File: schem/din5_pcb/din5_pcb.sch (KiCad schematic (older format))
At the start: 74 parts, among them J1 Conn_01x03_Male, J101 DIN-5_180degree, J102 DIN-5_180degree, J103 DIN-5_180degree, J104 DIN-5_180degree, J111 do not equip, J112 do not equip, J113 do not equip, J114 do not equip, J2 Conn_02x03_Odd_Even, J201 DIN-5_180degree, J202 DIN-5_180degree, J203 DIN-5_180degree, J204 DIN-5_180degree, J211 do not equip, J212 do not equip, J213 do not equip, J214 do not equip, J3 Conn_02x03_Odd_Even, J4 USB_B_Micro, J5 USB_B_Micro, J6 Conn_02x02_Odd_Even, J7 Conn_02x02_Odd_Even, U1 74HCT245, U101 HCPL-2630, U102 HCPL-2630, U2 74HC595, U3 74HC165

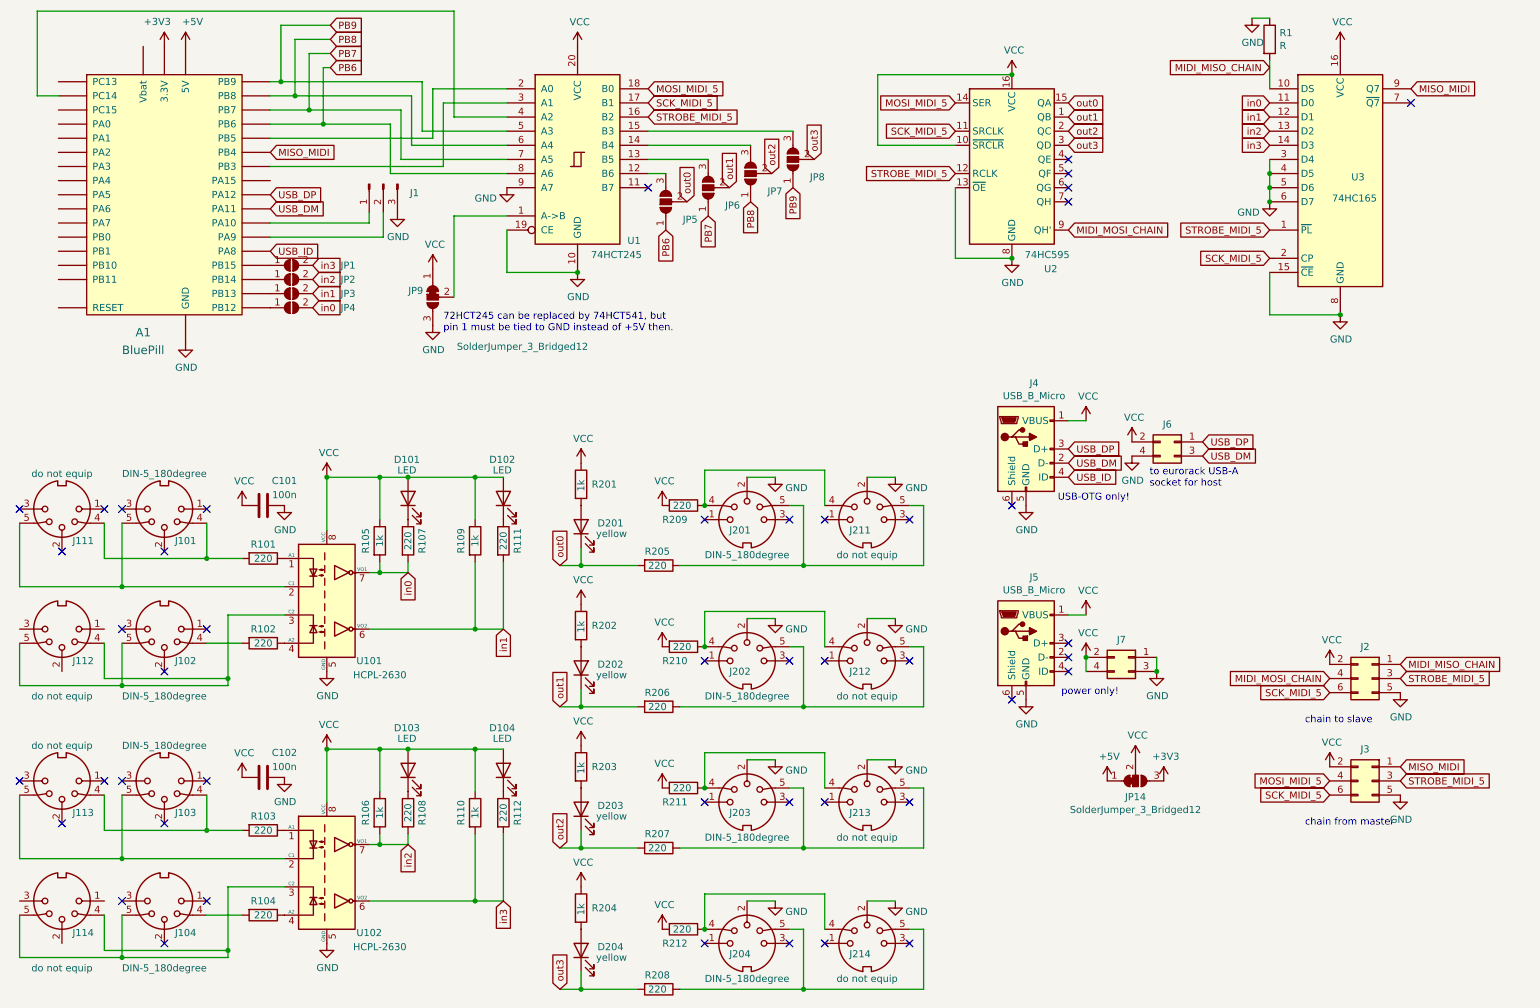
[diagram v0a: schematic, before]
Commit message: din 5 pin pcb finished. todo: autoroute
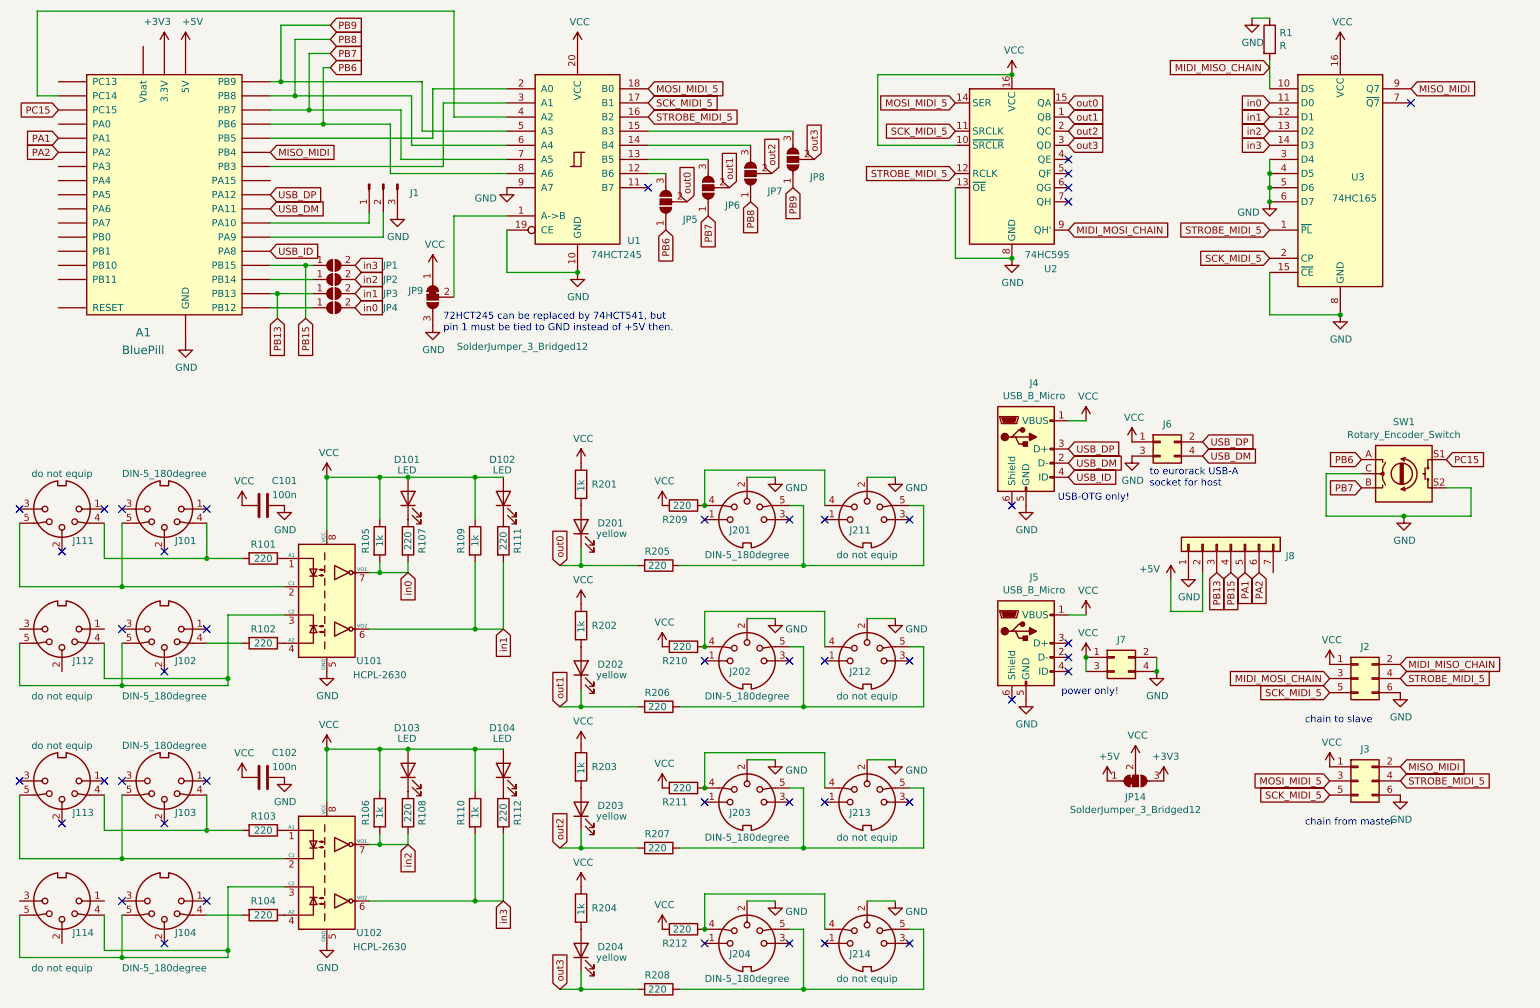
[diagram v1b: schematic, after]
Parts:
- added J8: Conn_01x07, Connector_PinHeader_2.54mm:PinHeader_1x07_P2.54mm_Vertical, symbol Connector_Generic:Conn_01x07
- added SW1: Rotary_Encoder_Switch, Rotary_Encoder:RotaryEncoder_Alps_EC11E-Switch_Vertical_H20mm, symbol Device:Rotary_Encoder_Switch
- J2, J3: footprint Connector_PinSocket_2.54mm:PinSocket_2x03_P2.54mm_Vertical -> Connector_PinHeader_2.54mm:PinHeader_2x03_P2.54mm_Vertical
- J6, J7: footprint Connector_PinSocket_2.54mm:PinSocket_2x02_P2.54mm_Vertical -> Connector_PinHeader_2.54mm:PinHeader_2x02_P2.54mm_Vertical
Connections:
- net +5V: now also J8.2 (Pin_2)
- net GND: now also J2.6 (Pin_6), J3.6 (Pin_6), J6.3 (Pin_3), J7.2 (Pin_2), J7.4 (Pin_4), J8.1 (Pin_1), SW1.C, SW1.S2; no longer J2.5 (Pin_5), J3.5 (Pin_5), J6.4 (Pin_4), J7.1 (Pin_1), J7.3 (Pin_3)
- net MIDI_MISO_CHAIN: now also J2.2 (Pin_2); no longer J2.1 (Pin_1)
- net MIDI_MOSI_CHAIN: now also J2.3 (Pin_3); no longer J2.4 (Pin_4)
- net MISO_MIDI: now also J3.2 (Pin_2); no longer J3.1 (Pin_1)
- net MOSI_MIDI_5: now also J3.3 (Pin_3); no longer J3.4 (Pin_4)
- net PB6: now also SW1.A
- net PB7: now also SW1.B
- net SCK_MIDI_5: now also J2.5 (Pin_5), J3.5 (Pin_5); no longer J2.6 (Pin_6), J3.6 (Pin_6)
- net STROBE_MIDI_5: now also J2.4 (Pin_4), J3.4 (Pin_4); no longer J2.3 (Pin_3), J3.3 (Pin_3)
- net USB_DM: now also J6.4 (Pin_4); no longer J6.3 (Pin_3)
- net USB_DP: now also J6.2 (Pin_2); no longer J6.1 (Pin_1)
- net VCC: now also J2.1 (Pin_1), J3.1 (Pin_1), J6.1 (Pin_1), J7.1 (Pin_1), J7.3 (Pin_3); no longer J2.2 (Pin_2), J3.2 (Pin_2), J6.2 (Pin_2), J7.2 (Pin_2), J7.4 (Pin_4)
- net PA1: now reaches A1.PA1
- net PA1: now also J8.5 (Pin_5)
- net PA2: now reaches A1.PA2
- net PA2: now also J8.6 (Pin_6)
- net PB13: now reaches A1.PB13, JP3.1 (A)
- net PB13: now also J8.3 (Pin_3)
- net PB15: now reaches A1.PB15, JP1.1 (A)
- net PB15: now also J8.4 (Pin_4)
- net PC15: now reaches A1.PC15
- net PC15: now also SW1.S1
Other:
- moved on the sheet: JP1, JP2, JP3, JP4
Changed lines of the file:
@@
 L Jumper:SolderJumper_2_Open JP4
 U 1 1 610951DC
-P 2450 2725
-F 0 "JP4" H 2850 2725 50  0000 C CNN
-F 1 "SolderJumper_2_Open" H 2450 2839 50  0001 C CNN
-F 2 "Jumper:SolderJumper-2_P1.3mm_Open_TrianglePad1.0x1.5mm" H 2450 2725 50  0001 C CNN
-F 3 "~" H 2450 2725 50  0001 C CNN
-	1    2450 2725
+P 2750 2725
+F 0 "JP4" H 3150 2725 50  0000 C CNN
+F 1 "SolderJumper_2_Open" H 2750 2839 50  0001 C CNN
+F 2 "Jumper:SolderJumper-2_P1.3mm_Open_TrianglePad1.0x1.5mm" H 2750 2725 50  0001 C CNN
+F 3 "~" H 2750 2725 50  0001 C CNN
+	1    2750 2725
 	1    0    0    -1
 $EndComp
@@
 L Jumper:SolderJumper_2_Open JP3
 U 1 1 610951D2
-P 2450 2625
-F 0 "JP3" H 2850 2625 50  0000 C CNN
-F 1 "SolderJumper_2_Open" H 2450 2739 50  0001 C CNN
-F 2 "Jumper:SolderJumper-2_P1.3mm_Open_TrianglePad1.0x1.5mm" H 2450 2625 50  0001 C CNN
-F 3 "~" H 2450 2625 50  0001 C CNN
-	1    2450 2625
+P 2750 2625
+F 0 "JP3" H 3150 2625 50  0000 C CNN
+F 1 "SolderJumper_2_Open" H 2750 2739 50  0001 C CNN
+F 2 "Jumper:SolderJumper-2_P1.3mm_Open_TrianglePad1.0x1.5mm" H 2750 2625 50  0001 C CNN
+F 3 "~" H 2750 2625 50  0001 C CNN
+	1    2750 2625
 	1    0    0    -1
 $EndComp
@@
 L Jumper:SolderJumper_2_Open JP2
 U 1 1 610951C8
-P 2450 2525
-F 0 "JP2" H 2850 2525 50  0000 C CNN
-F 1 "SolderJumper_2_Open" H 2450 2639 50  0001 C CNN
-F 2 "Jumper:SolderJumper-2_P1.3mm_Open_TrianglePad1.0x1.5mm" H 2450 2525 50  0001 C CNN
-F 3 "~" H 2450 2525 50  0001 C CNN
-	1    2450 2525
+P 2750 2525
+F 0 "JP2" H 3150 2525 50  0000 C CNN
+F 1 "SolderJumper_2_Open" H 2750 2639 50  0001 C CNN
+F 2 "Jumper:SolderJumper-2_P1.3mm_Open_TrianglePad1.0x1.5mm" H 2750 2525 50  0001 C CNN
+F 3 "~" H 2750 2525 50  0001 C CNN
+	1    2750 2525
 	1    0    0    -1
 $EndComp
@@
 L Jumper:SolderJumper_2_Open JP1
 U 1 1 61094C0C
-P 2450 2425
-F 0 "JP1" H 2850 2425 50  0000 C CNN
-F 1 "SolderJumper_2_Open" H 2450 2539 50  0001 C CNN
-F 2 "Jumper:SolderJumper-2_P1.3mm_Open_TrianglePad1.0x1.5mm" H 2450 2425 50  0001 C CNN
-F 3 "~" H 2450 2425 50  0001 C CNN
-	1    2450 2425
+P 2750 2425
+F 0 "JP1" H 3150 2425 50  0000 C CNN
+F 1 "SolderJumper_2_Open" H 2750 2539 50  0001 C CNN
+F 2 "Jumper:SolderJumper-2_P1.3mm_Open_TrianglePad1.0x1.5mm" H 2750 2425 50  0001 C CNN
+F 3 "~" H 2750 2425 50  0001 C CNN
+	1    2750 2425
 	1    0    0    -1
 $EndComp
@@
 	1    0    0    -1
 $EndComp
-Text GLabel 2600 2425 2    50   Input ~ 0
+Text GLabel 2900 2425 2    50   Input ~ 0
 in3
-Text GLabel 2600 2525 2    50   Input ~ 0
+Text GLabel 2900 2525 2    50   Input ~ 0
 in2
-Text GLabel 2600 2625 2    50   Input ~ 0
+Text GLabel 2900 2625 2    50   Input ~ 0
 in1
-Text GLabel 2600 2725 2    50   Input ~ 0
+Text GLabel 2900 2725 2    50   Input ~ 0
 in0
 Wire Wire Line
@@
 L Connector_Generic:Conn_02x03_Odd_Even J2
 U 1 1 60E04254
-P 10100 5350
-F 0 "J2" H 10150 5575 50  0000 C CNN
-F 1 "Conn_02x03_Odd_Even" H 10150 5576 50  0001 C CNN
-F 2 "Connector_PinSocket_2.54mm:PinSocket_2x03_P2.54mm_Vertical" H 10100 5350 50  0001 C CNN
-F 3 "~" H 10100 5350 50  0001 C CNN
-	1    10100 5350
-	-1   0    0    -1
+P 10000 5350
+F 0 "J2" H 10050 5575 50  0000 C CNN
+F 1 "Conn_02x03_Odd_Even" H 10050 5576 50  0001 C CNN
+F 2 "Connector_PinHeader_2.54mm:PinHeader_2x03_P2.54mm_Vertical" H 10000 5350 50  0001 C CNN
+F 3 "~" H 10000 5350 50  0001 C CNN
+	1    10000 5350
+	1    0    0    -1
 $EndComp
 $Comp
 L Connector_Generic:Conn_02x03_Odd_Even J3
 U 1 1 60E118D4
-P 10100 6075
-F 0 "J3" H 10150 6300 50  0000 C CNN
-F 1 "Conn_02x03_Odd_Even" H 10150 6301 50  0001 C CNN
-F 2 "Connector_PinSocket_2.54mm:PinSocket_2x03_P2.54mm_Vertical" H 10100 6075 50  0001 C CNN
-F 3 "~" H 10100 6075 50  0001 C CNN
-	1    10100 6075
-	-1   0    0    -1
+P 10000 6075
+F 0 "J3" H 10050 6300 50  0000 C CNN
+F 1 "Conn_02x03_Odd_Even" H 10050 6301 50  0001 C CNN
+F 2 "Connector_PinHeader_2.54mm:PinHeader_2x03_P2.54mm_Vertical" H 10000 6075 50  0001 C CNN
+F 3 "~" H 10000 6075 50  0001 C CNN
+	1    10000 6075
+	1    0    0    -1
 $EndComp
 $Comp
 L Connector_Generic:Conn_02x02_Odd_Even J7
 U 1 1 60E1FECA
-P 8375 5200
-F 0 "J7" H 8425 5325 50  0000 C CNN
-F 1 "Conn_02x02_Odd_Even" H 8425 5326 50  0001 C CNN
-F 2 "Connector_PinSocket_2.54mm:PinSocket_2x02_P2.54mm_Vertical" H 8375 5200 50  0001 C CNN
-F 3 "~" H 8375 5200 50  0001 C CNN
-	1    8375 5200
-	-1   0    0    -1
-$EndComp
+P 8275 5200
+F 0 "J7" H 8325 5325 50  0000 C CNN
+F 1 "Conn_02x02_Odd_Even" H 8325 5326 50  0001 C CNN
+F 2 "Connector_PinHeader_2.54mm:PinHeader_2x02_P2.54mm_Vertical" H 8275 5200 50  0001 C CNN
+F 3 "~" H 8275 5200 50  0001 C CNN
+	1    8275 5200
+	1    0    0    -1
+$EndComp
+Connection ~ 8075 5200
+Connection ~ 8575 5300
 $Comp
 L Connector_Generic:Conn_02x02_Odd_Even J6
 U 1 1 60E2ACED
-P 8700 3675
-F 0 "J6" H 8750 3800 50  0000 C CNN
-F 1 "Conn_02x02_Odd_Even" H 8750 3801 50  0001 C CNN
-F 2 "Connector_PinSocket_2.54mm:PinSocket_2x02_P2.54mm_Vertical" H 8700 3675 50  0001 C CNN
-F 3 "~" H 8700 3675 50  0001 C CNN
-	1    8700 3675
-	-1   0    0    -1
-$EndComp
-Connection ~ 8075 5200
-Connection ~ 8575 5300
+P 8600 3675
+F 0 "J6" H 8650 3800 50  0000 C CNN
+F 1 "Conn_02x02_Odd_Even" H 8650 3801 50  0001 C CNN
+F 2 "Connector_PinHeader_2.54mm:PinHeader_2x02_P2.54mm_Vertical" H 8600 3675 50  0001 C CNN
+F 3 "~" H 8600 3675 50  0001 C CNN
+	1    8600 3675
+	1    0    0    -1
+$EndComp
+$Comp
+L Device:Rotary_Encoder_Switch SW1
+U 1 1 60F5FE54
+P 10325 3900
+F 0 "SW1" H 10325 4267 50  0000 C CNN
+F 1 "Rotary_Encoder_Switch" H 10325 4176 50  0000 C CNN
+F 2 "Rotary_Encoder:RotaryEncoder_Alps_EC11E-Switch_Vertical_H20mm" H 10175 4060 50  0001 C CNN
+F 3 "~" H 10325 4160 50  0001 C CNN
+	1    10325 3900
+	1    0    0    -1
+$EndComp
+Wire Wire Line
+	10025 3900 9775 3900
+Wire Wire Line
+	9775 3900 9775 4200
+Wire Wire Line
+	9775 4200 10325 4200
+Wire Wire Line
+	10800 4200 10800 4000
+Wire Wire Line
+	10800 4000 10625 4000
+$Comp
+L power:GND #PWR024
+U 1 1 60F9A317
+P 10325 4200
+F 0 "#PWR024" H 10325 3950 50  0001 C CNN
+F 1 "GND" H 10330 4027 50  0000 C CNN
+F 2 "" H 10325 4200 50  0001 C CNN
+F 3 "" H 10325 4200 50  0001 C CNN
+	1    10325 4200
+	1    0    0    -1
+$EndComp
+Connection ~ 10325 4200
+Wire Wire Line
+	10325 4200 10800 4200
+Text GLabel 10025 3800 0    50   Input ~ 0
+PB6
+Text GLabel 10025 4000 0    50   Input ~ 0
+PB7
+Text GLabel 10625 3800 2    50   Input ~ 0
+PC15
+Text GLabel 800  1325 0    50   Input ~ 0
+PC15
+$Comp
+L Connector_Generic:Conn_01x07 J8
+U 1 1 60FCFEC2
+P 9100 4400
+F 0 "J8" V 9018 4012 50  0000 R CNN
+F 1 "Conn_01x07" V 8973 4012 50  0001 R CNN
+F 2 "Connector_PinHeader_2.54mm:PinHeader_1x07_P2.54mm_Vertical" H 9100 4400 50  0001 C CNN
+F 3 "~" H 9100 4400 50  0001 C CNN
+	1    9100 4400
+	0    -1   -1   0
+$EndComp
+Text GLabel 2350 2800 3    50   Input ~ 0
+PB13
+Wire Wire Line
+	2300 2425 2550 2425
+Wire Wire Line
+	2600 2625 2350 2625
+Wire Wire Line
+	2300 2725 2600 2725
+Wire Wire Line
+	2350 2800 2350 2625
+Connection ~ 2350 2625
+Wire Wire Line
+	2350 2625 2300 2625
+Text GLabel 2550 2800 3    50   Input ~ 0
+PB15
+Wire Wire Line
+	2550 2800 2550 2425
+Connection ~ 2550 2425
+Wire Wire Line
+	2550 2425 2600 2425
+Text GLabel 9000 4600 3    50   Input ~ 0
+PB13
+Text GLabel 9100 4600 3    50   Input ~ 0
+PB15
+$Comp
+L power:GND #PWR023
+U 1 1 6105C50C
+P 8800 4600
+F 0 "#PWR023" H 8800 4350 50  0001 C CNN
+F 1 "GND" H 8805 4427 50  0000 C CNN
+F 2 "" H 8800 4600 50  0001 C CNN
+F 3 "" H 8800 4600 50  0001 C CNN
+	1    8800 4600
+	1    0    0    -1
+$EndComp
+Wire Wire Line
+	8900 4600 8900 4875
+Wire Wire Line
+	8900 4875 8675 4875
+Wire Wire Line
+	8675 4875 8675 4650
+$Comp
+L power:+5V #PWR05
+U 1 1 6106B5E8
+P 8675 4650
+F 0 "#PWR05" H 8675 4500 50  0001 C CNN
+F 1 "+5V" H 8525 4725 50  0000 C CNN
+F 2 "" H 8675 4650 50  0001 C CNN
+F 3 "" H 8675 4650 50  0001 C CNN
+	1    8675 4650
+	1    0    0    -1
+$EndComp
+Wire Wire Line
+	2300 2525 2600 2525
+Text GLabel 800  1525 0    50   Input ~ 0
+PA1
+Text GLabel 800  1625 0    50   Input ~ 0
+PA2
+Text GLabel 9200 4600 3    50   Input ~ 0
+PA1
+Text GLabel 9300 4600 3    50   Input ~ 0
+PA2
 $EndSCHEMATC
